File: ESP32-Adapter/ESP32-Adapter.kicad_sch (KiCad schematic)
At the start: 20 parts, among them J1 Conn_01x01_Socket, J12 Conn_01x05, J13 Conn_01x05, J14 Conn_01x04, J2 Conn_01x03, J3 Conn_01x03, J4 Conn_01x01_Socket, J5 Conn_01x01_Socket, J6 Conn_01x01_Socket, J7 Conn_01x01_Socket, J8 Conn_01x01_Socket, J9 Conn_01x01_Socket, U1 ESP32-C5-DevKitC-1, U2 LM317_TO-263, U3 Adafruit CANPAL

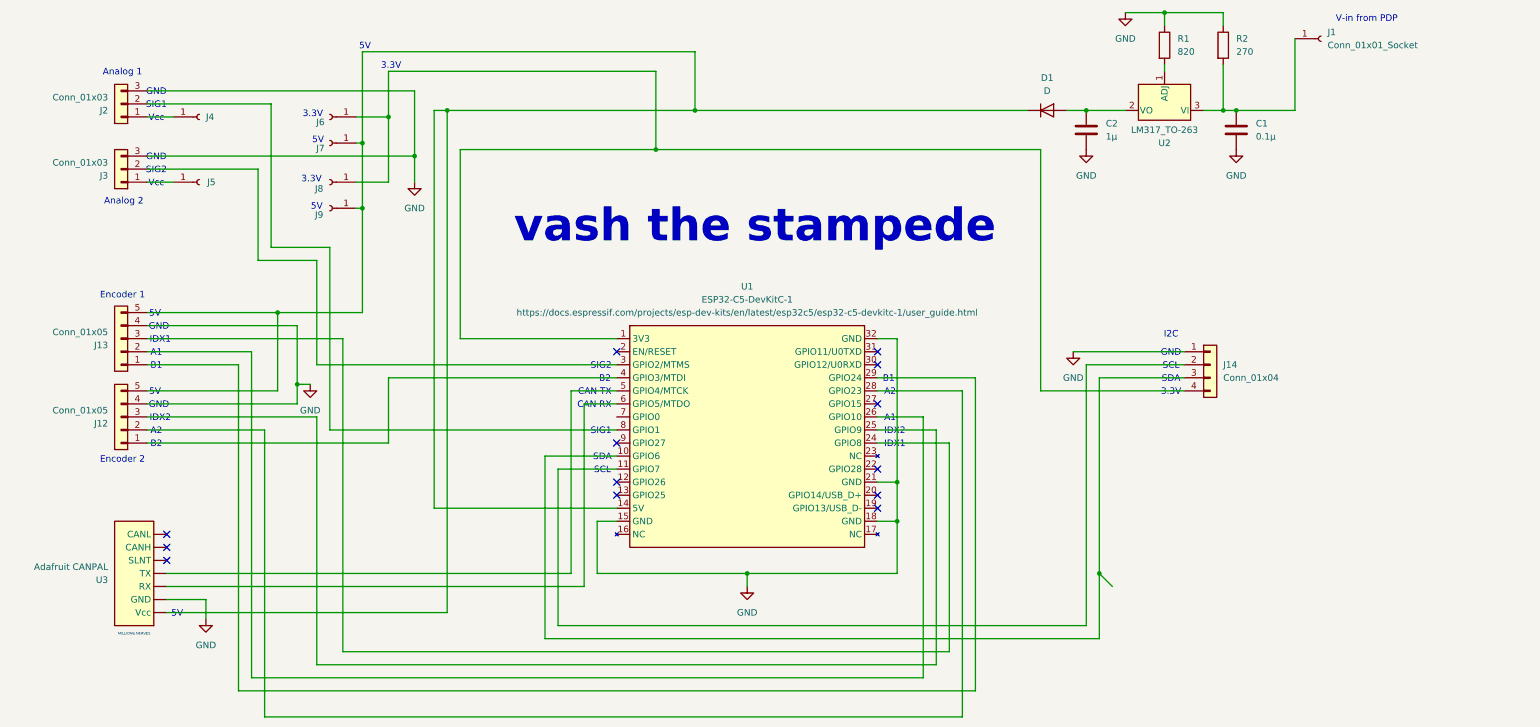
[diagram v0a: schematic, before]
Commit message: create pcb
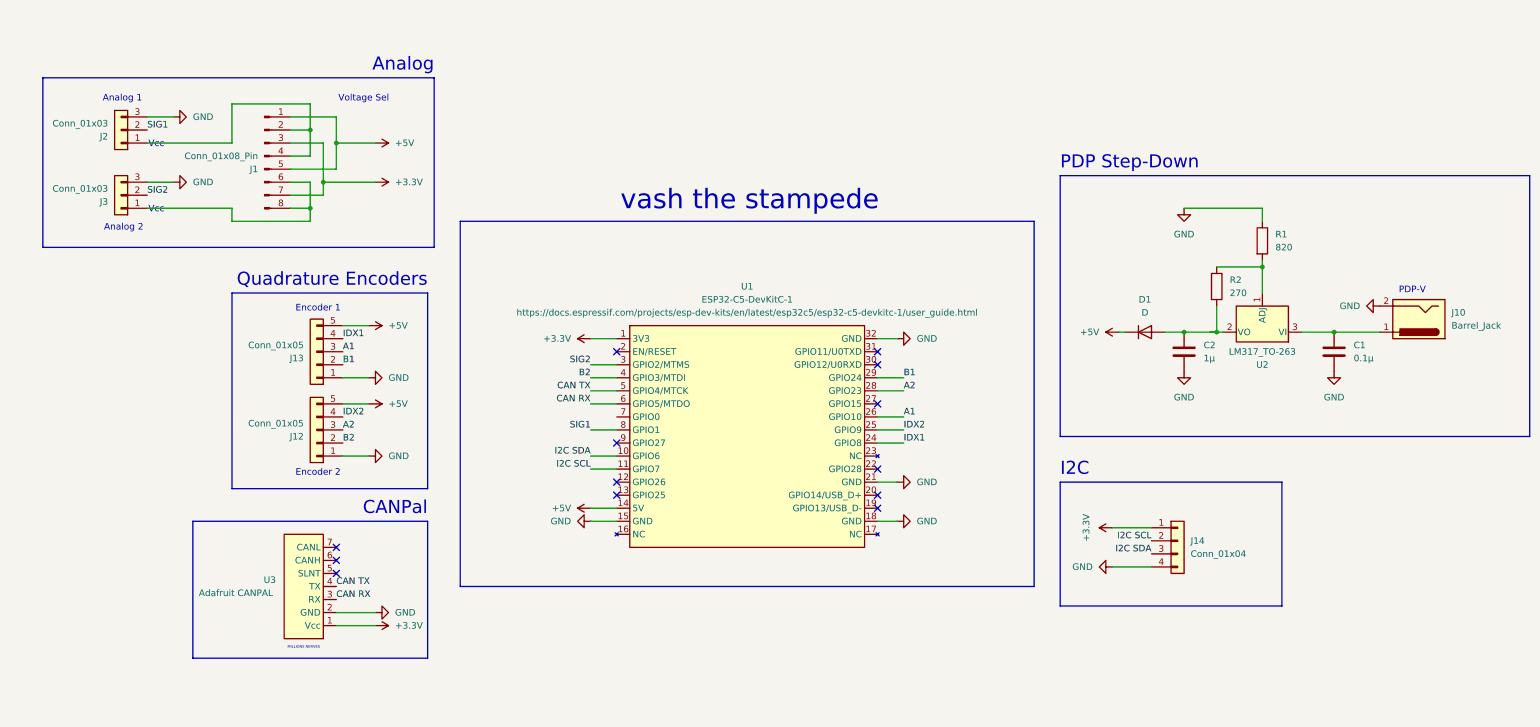
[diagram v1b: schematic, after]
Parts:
- removed J1, J4, J5, J6, J7, J8, J9: Conn_01x01_Socket, symbol Connector:Conn_01x01_Socket
- added J1: Conn_01x08_Pin, Connector_PinHeader_2.54mm:PinHeader_2x04_P2.54mm_Vertical, symbol Connector:Conn_01x08_Pin
- added J10: Barrel_Jack, Connector_BarrelJack:BarrelJack_CUI_PJ-063AH_Horizontal, symbol Connector:Barrel_Jack
- C1, C2: footprint (none) -> Capacitor_SMD:C_0402_1005Metric
- D1: footprint (none) -> Diode_SMD:D_0805_2012Metric
- J12, J13: footprint (none) -> Connector_JST:JST_XH_S5B-XH-A-1_1x05_P2.50mm_Horizontal
- J14: footprint (none) -> Connector_JST:JST_XH_S4B-XH-A-1_1x04_P2.50mm_Horizontal
- J2, J3: footprint (none) -> Connector_JST:JST_XH_S3B-XH-A-1_1x03_P2.50mm_Horizontal
- R1, R2: footprint (none) -> Resistor_SMD:R_0402_1005Metric
- U3: footprint (none) -> Audio_Module:canpal
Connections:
- net GND: now also J12.1 (Pin_1), J13.1 (Pin_1), J14.4 (Pin_4), U3.2 (GND), J10.2; no longer J12.4 (Pin_4), J13.4 (Pin_4), J14.1 (Pin_1), R2.1, U3. (CANL)
- net at J3.1 (Pin_1): now also J1.6 (Pin_6), J1.8 (Pin_8)
- net I2C SCL: now reaches J14.2 (Pin_2), U1.11 (GPIO7)
- net I2C SDA: now reaches J14.3 (Pin_3), U1.10 (GPIO6)
- net +3.3V: now reaches U1.1 (3V3)
- net +3.3V: now also J14.1 (Pin_1), U3.1 (Vcc), J1.3 (Pin_3), J1.7 (Pin_7); no longer J14.4 (Pin_4)
- net at C2.1, D1.2 (A), U2.2 (VO): now also R2.2
- net at C1.1, U2.3 (VI): now also J10.1; no longer R2.2
- net B2: now reaches U1.4 (GPIO3/MTDI)
- net B2: now also J12.2 (Pin_2); no longer J12.1 (Pin_1)
- net A2: now reaches U1.28 (GPIO23)
- net A2: now also J12.3 (Pin_3); no longer J12.2 (Pin_2)
- net IDX2: now reaches U1.25 (GPIO9)
- net IDX2: now also J12.4 (Pin_4); no longer J12.3 (Pin_3)
- net +5V: now reaches D1.1 (K), J12.5 (Pin_5), J13.5 (Pin_5), U1.14 (5V)
- net +5V: now also J1.1 (Pin_1), J1.5 (Pin_5); no longer U3. (CANL)
- net SIG2: now reaches J3.2 (Pin_2), U1.3 (GPIO2/MTMS)
- net at R1.2, U2.1 (ADJ): now also R2.1
- net B1: now reaches U1.29 (GPIO24)
- net B1: now also J13.2 (Pin_2); no longer J13.1 (Pin_1)
- net A1: now reaches U1.26 (GPIO10)
- net A1: now also J13.3 (Pin_3); no longer J13.2 (Pin_2)
- net IDX1: now reaches U1.24 (GPIO8)
- net IDX1: now also J13.4 (Pin_4); no longer J13.3 (Pin_3)
- net CAN TX: now reaches U1.5 (GPIO4/MTCK)
- net CAN TX: now also U3.4 (TX); no longer U3. (CANL)
- net CAN RX: now reaches U1.6 (GPIO5/MTDO)
- net CAN RX: now also U3.3 (RX); no longer U3. (CANL)
- net SIG1: now reaches J2.2 (Pin_2), U1.8 (GPIO1)
- net at J2.1 (Pin_1): now also J1.2 (Pin_2), J1.4 (Pin_4)
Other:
- note added: "Analog"
- note added: "CANPal"
- note added: "PDP Step-Down"
- note added: "PDP-V"
- note added: "Quadrature Encoders"
- note added: "Voltage Sel"
- note removed: "3.3V"
- note removed: "5V"
- note removed: "A1"
- note removed: "A2"
- note removed: "B1"
- note removed: "B2"
- note removed: "CAN RX"
- note removed: "CAN TX"
- note removed: "GND"
- note removed: "IDX1"
- note removed: "IDX2"
- note removed: "SCL"
- note removed: "SDA"
- note removed: "SIG1"
- note removed: "SIG2"
- note removed: "V-in from PDP"
- moved on the sheet: C1, C2, D1, J12, J13, J14, J2, J3, R1, R2, U2
